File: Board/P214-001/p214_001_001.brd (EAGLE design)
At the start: 70.8 x 71.1 mm, 23 parts, among them IC1 74LS07N

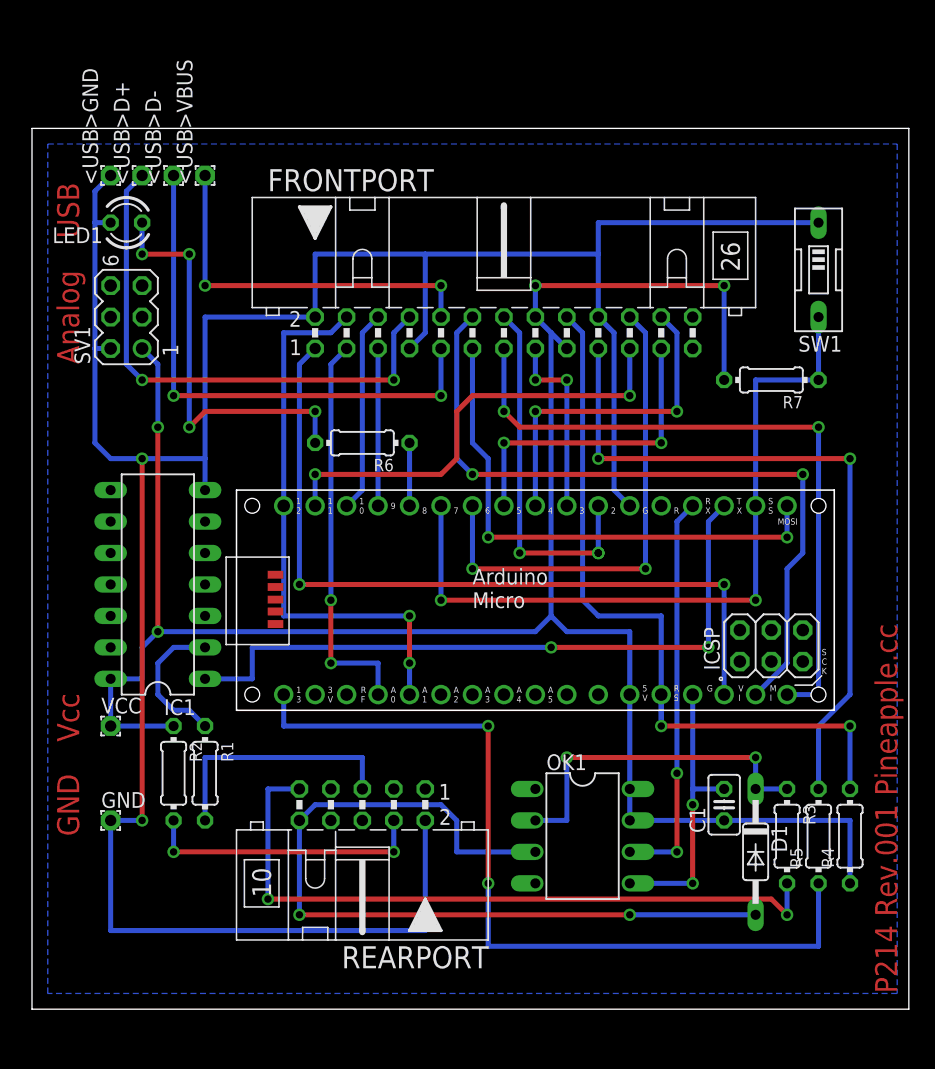
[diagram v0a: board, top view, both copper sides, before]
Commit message: new design.
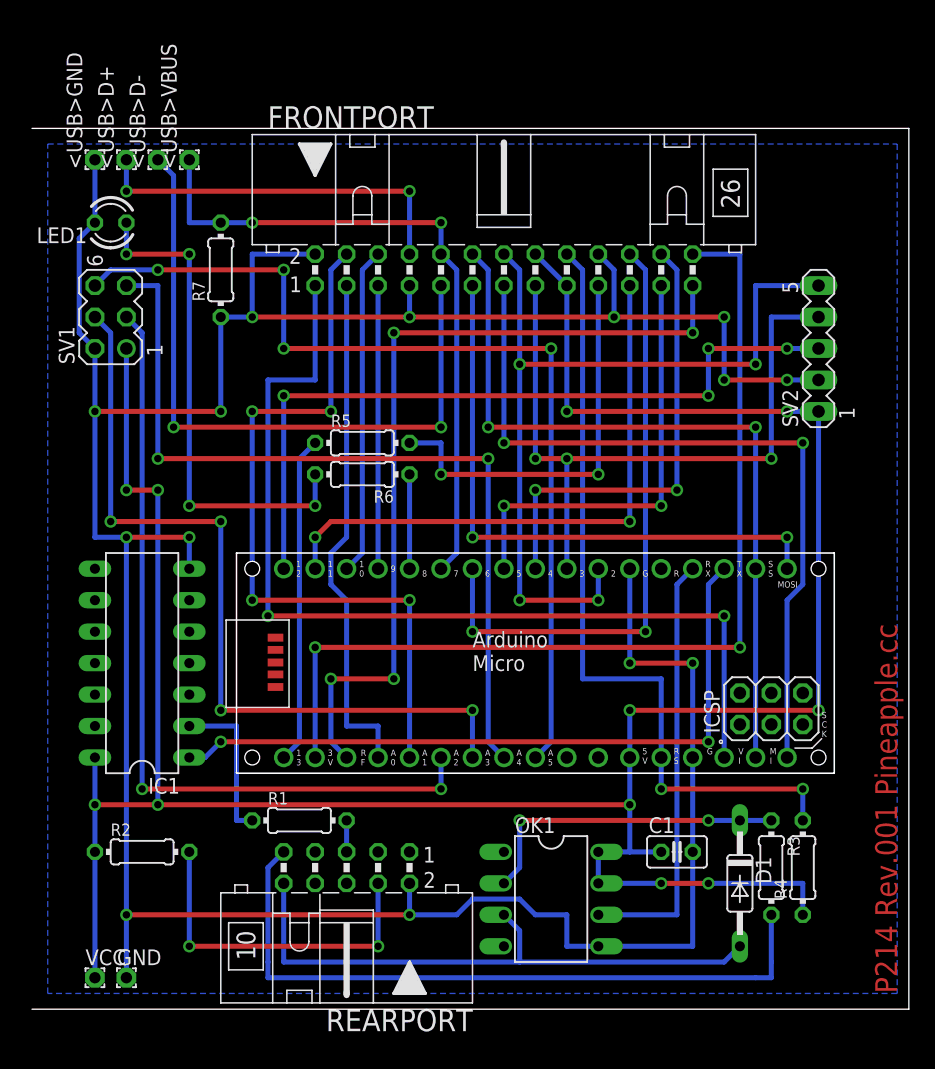
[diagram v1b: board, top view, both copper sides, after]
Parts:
- removed SW1: (no value), special:EDG-01
- added SV2: (no value), con-lstb:MA05-1
- C1: value (none) -> 104
- R4: value (none) -> 10k
- R5, R6: value (none) -> 300
- moved R5 48.6 mm to (26.7, 45.7), turned to 0 degrees
- moved R7 45.3 mm to (15.2, 59.7), turned to 90 degrees
- moved VCC 20.4 mm to (5.08, 2.54)
- moved GND 12.8 mm to (7.62, 2.54)
- moved R1 8.52 mm to (21.6, 15.2), turned to 0 degrees
- moved R2 6.84 mm to (8.89, 12.7), turned to 0 degrees
- moved IC1 6.48 mm to (8.89, 27.9)
- moved OK1 5.68 mm to (41.9, 8.89)
- moved C1 5.39 mm to (52.1, 12.7), turned to 0 degrees
- moved REARPORT 5.24 mm to (25.4, 11.4)
- moved FRONTPORT 5.08 mm to (38.1, 59.7)
- moved PCB1 5.08 mm to (16.5, 19.1)
- moved R4 4.58 mm to (62.2, 11.4)
- moved R3 2.84 mm to (59.7, 11.4)
- moved D1 2.84 mm to (57.1, 10.2)
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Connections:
- net GND: now also R7.1, SV2.2; no longer SW1.1
- net N$17: now also SV2.5
- net N$18: now also SV2.4
- net N$25: now also PCB1.D7, R7.2
- net N$37: now also PCB1.D12, SV2.3; no longer PCB1.D7, R7.1, SW1.2
- net VCC: now also SV2.1; no longer R7.2
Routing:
- net N$30: track 0.00 -> 78.7 mm, vias 0 -> 2
- net N$34: track 0.00 -> 77.3 mm, vias 0 -> 4
- net N$21: track 0.00 -> 67.8 mm, vias 0 -> 4
- net N$33: track 0.00 -> 67.8 mm, vias 0 -> 2
- net N$32: track 0.00 -> 65.3 mm, vias 0 -> 4
- net N$31: track 0.00 -> 65.3 mm, vias 0 -> 2
- net VCC: track 168.3 -> 211.9 mm, vias 4 -> 11
- net N$20: track 68.6 -> 26.5 mm, vias 2 -> 0
- net N$18: track 15.2 -> 57.1 mm, vias 2 -> 3
- net N$17: track 29.7 -> 67.8 mm, vias 3 -> 4
- net N$19: track 56.9 -> 33.0 mm
- net N$25: track 30.5 -> 54.4 mm
- net GND: track 232.5 -> 254.1 mm, vias 4 -> 15
- net N$7: track 67.1 -> 48.0 mm, vias 2 -> 0
- net N$5: track 20.3 -> 2.54 mm
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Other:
- board text removed: "Analog"
- board text removed: "GND"
- board text removed: "USB"
- board text removed: "Vcc"
